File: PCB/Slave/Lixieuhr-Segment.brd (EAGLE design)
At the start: 45 x 65 mm, 50 parts, among them U1 APA102C, U10 APA102C, U11 APA102C, U12 APA102C, U13 APA102C, U14 APA102C, U15 APA102C, U16 APA102C, U17 APA102C, U18 APA102C, U19 APA102C, U2 APA102C, U20 APA102C, U3 APA102C, U4 APA102C, U5 APA102C, U6 APA102C, U7 APA102C, U8 APA102C, U9 APA102C

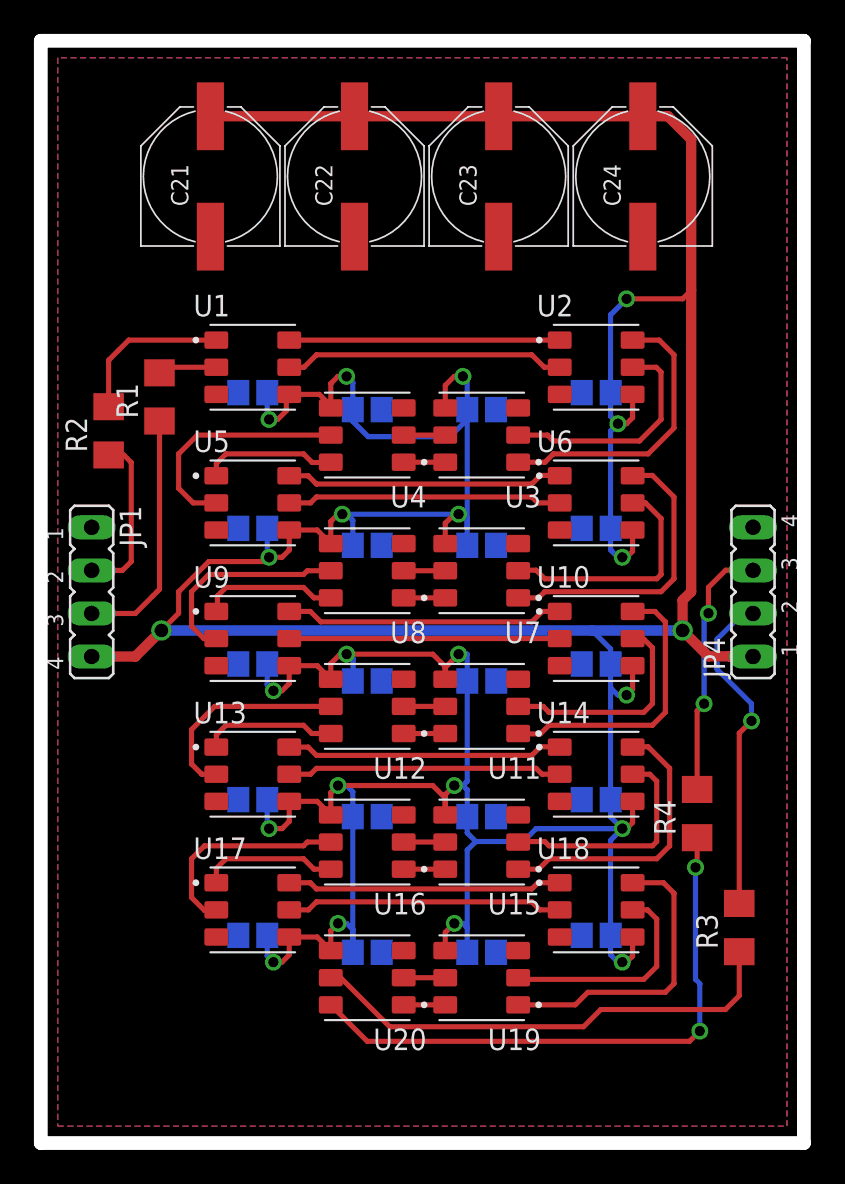
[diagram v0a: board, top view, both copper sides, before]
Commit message: V05
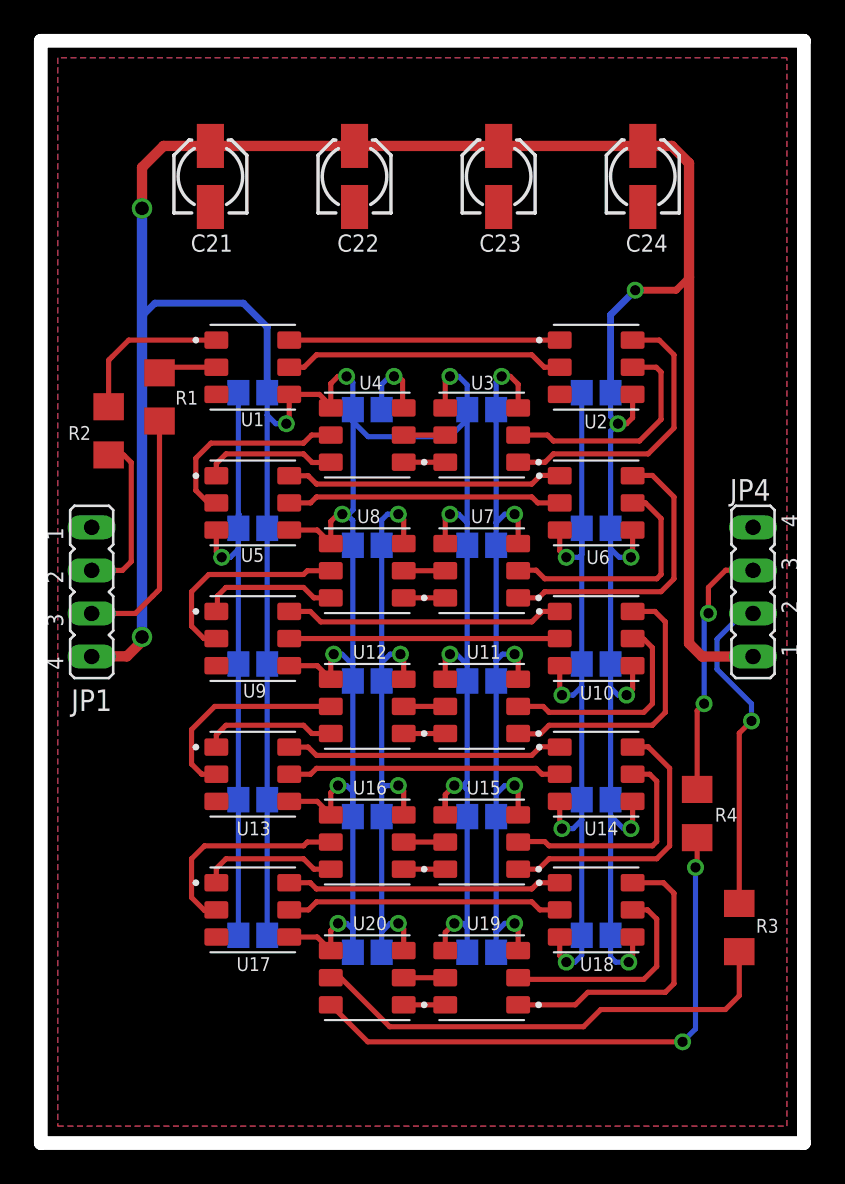
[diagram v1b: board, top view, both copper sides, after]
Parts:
- C21, C22, C23, C24: device 0_HTL_MegaCard_V3:PANASONIC_F -> resistor:153CLV-0405
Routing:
- net GND: track 0.00 -> 174.9 mm, vias 0 -> 15
- net V+: track 304.8 -> 325.6 mm, vias 23 -> 19
- net N$4: track 14.0 -> 11.9 mm
